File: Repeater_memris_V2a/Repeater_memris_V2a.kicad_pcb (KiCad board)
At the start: 4 copper layers, 96 x 83 mm, 73 parts, among them J2 Conn_01x06_Socket, Q1 MMBT2222A, Q2 MMBT2222A, U1 ATmega328-A, U2 AMS1117-3.3, U3 SA868-U, U4 SA868-V, U5 4016, U6 SPF5043Z, Y1 Crystal_GND2

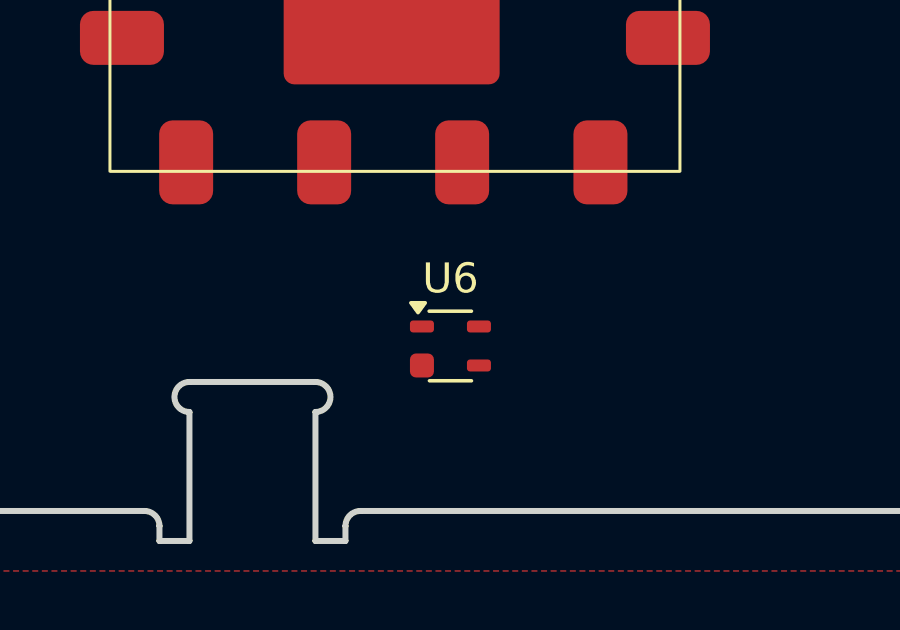
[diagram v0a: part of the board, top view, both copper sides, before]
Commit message: Revert "sch pcb update"
This reverts commit 82fe7de560fbc9173e196ee1871e922f74af1bd5.
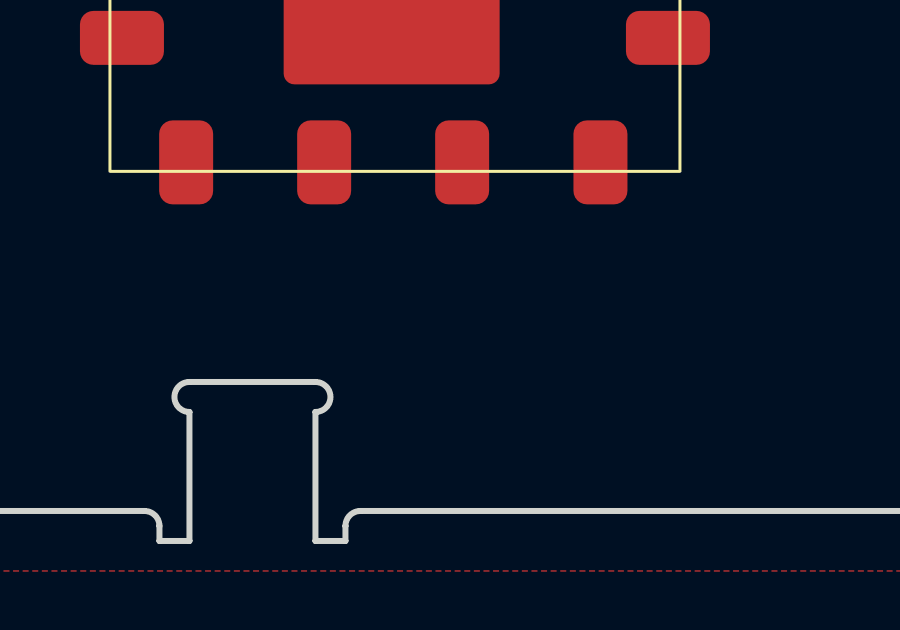
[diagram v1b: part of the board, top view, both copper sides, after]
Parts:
- removed U6: SPF5043Z, Package_TO_SOT_SMD:SOT-343_SC-70-4
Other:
- copper layers 4 -> 2

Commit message: sch pcb update
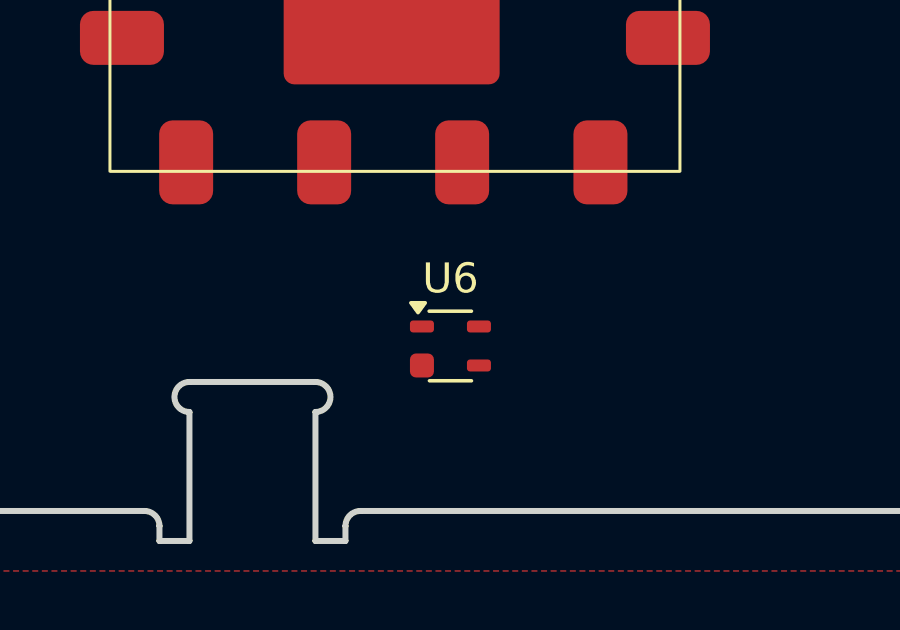
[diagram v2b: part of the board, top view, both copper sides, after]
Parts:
- added U6: SPF5043Z, Package_TO_SOT_SMD:SOT-343_SC-70-4, F.Cu at (124.5, 135.5)
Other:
- copper layers 2 -> 4
